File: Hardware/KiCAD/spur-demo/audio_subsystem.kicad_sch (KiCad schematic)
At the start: 16 parts, among them U3 MAX98357A, U4 LM393

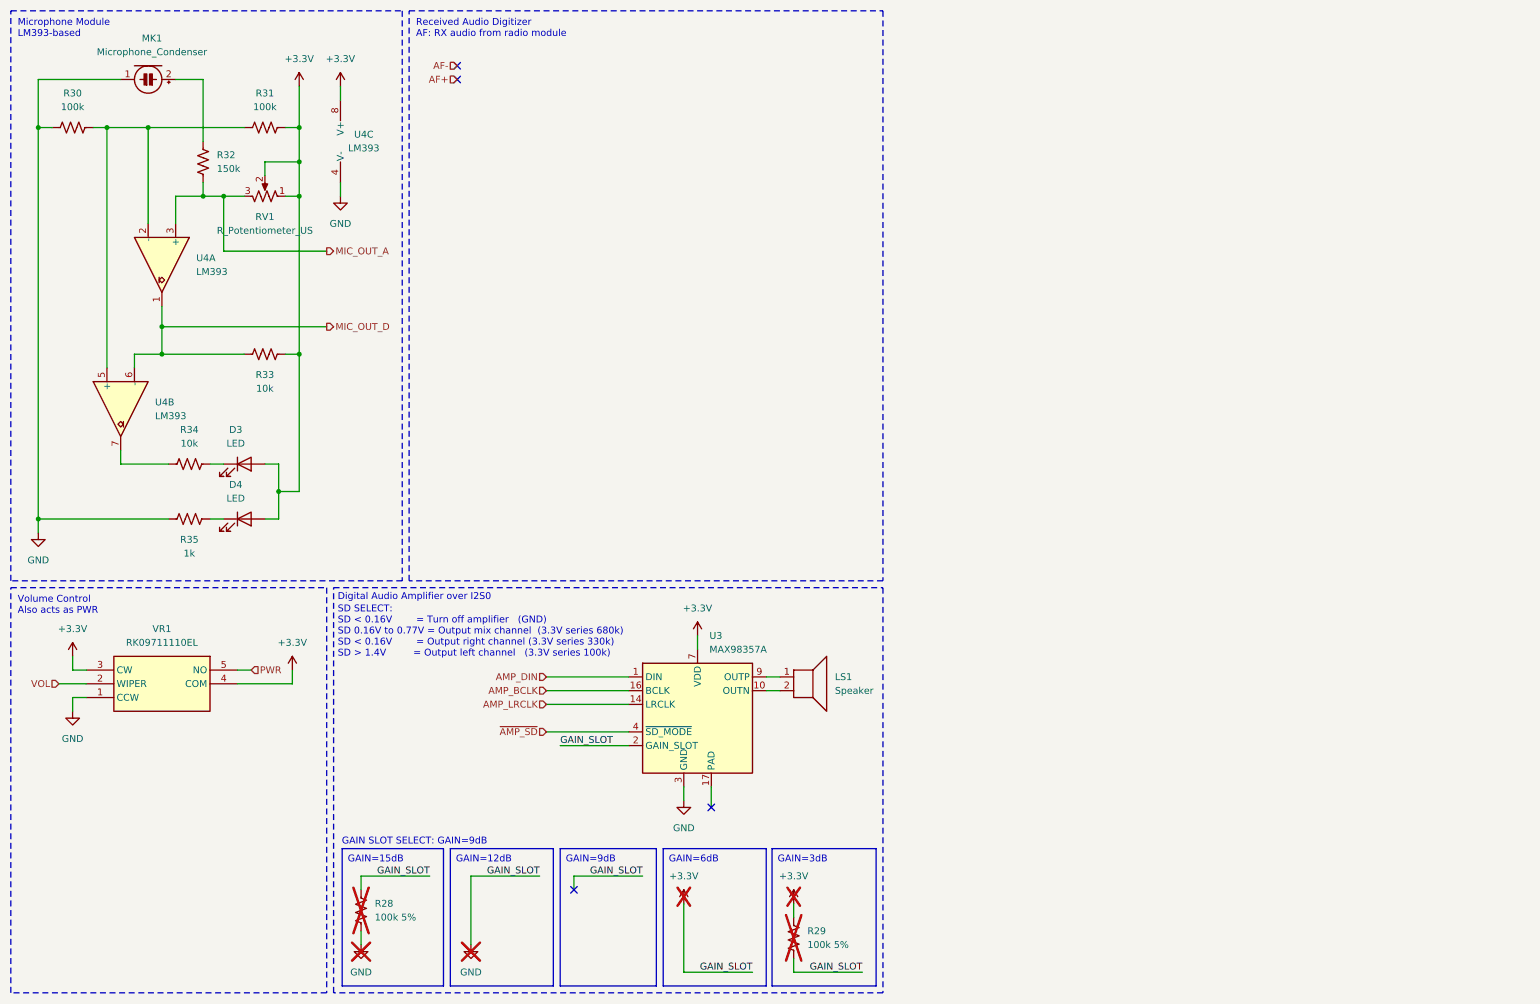
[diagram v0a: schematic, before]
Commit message: feat: configuration for audio amp through solder jumpers with set defaults
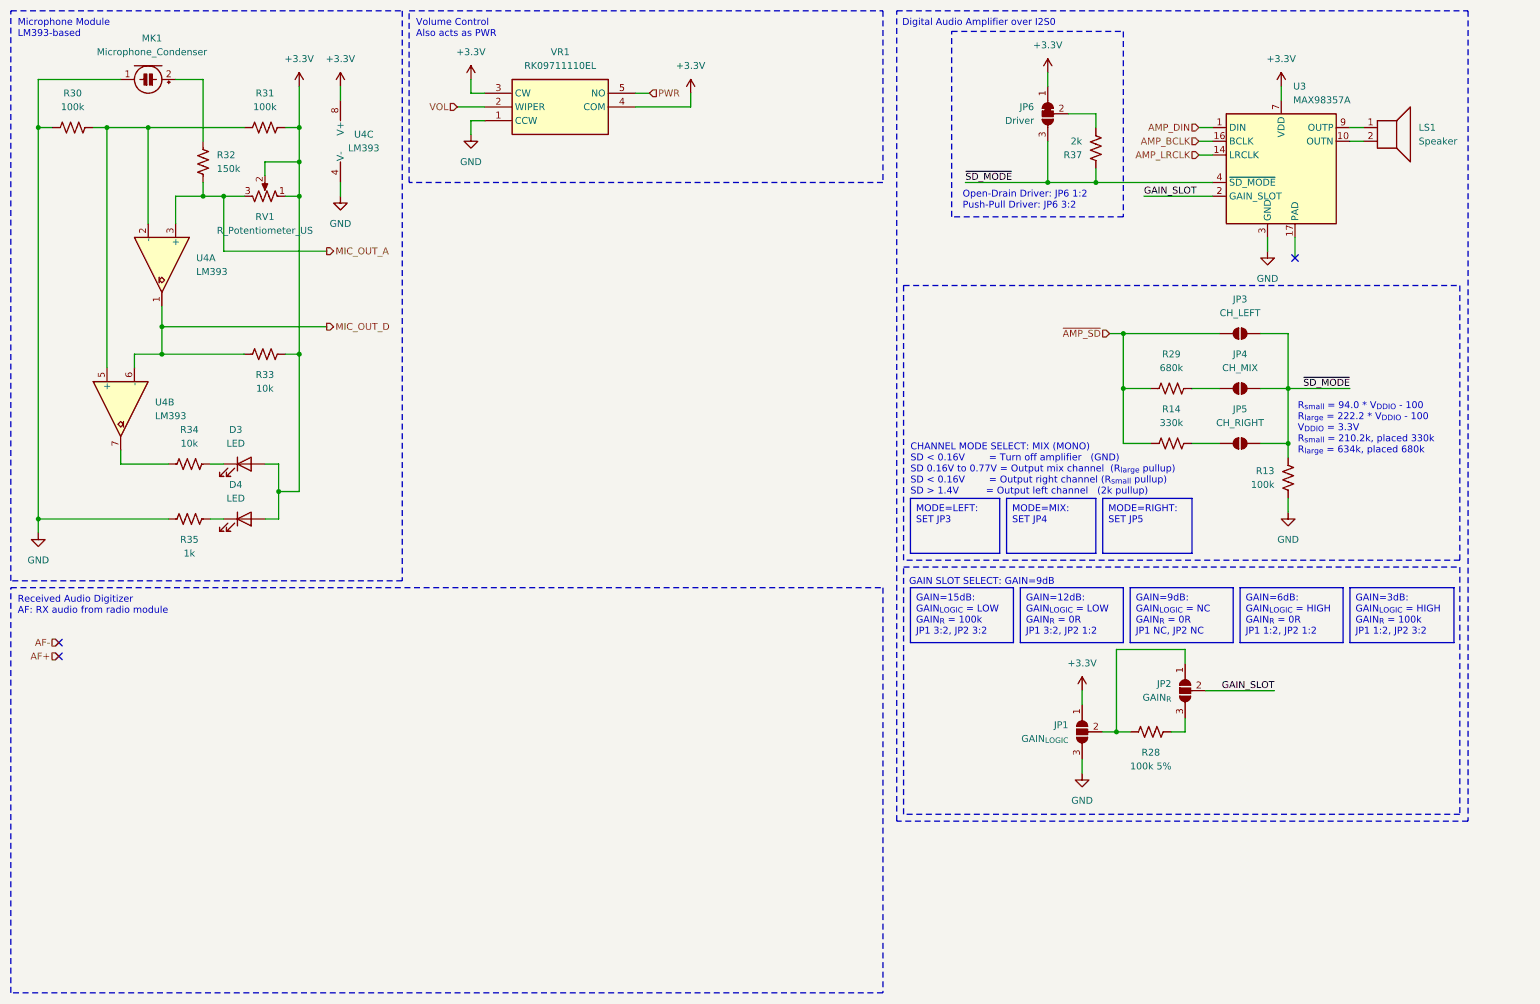
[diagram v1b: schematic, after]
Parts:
- added JP1: GAIN_{LOGIC}, symbol Jumper:SolderJumper_3_Open
- added JP2: GAIN_{R}, symbol Jumper:SolderJumper_3_Open
- added JP3: CH_LEFT, symbol Jumper:SolderJumper_2_Open
- added JP4: CH_MIX, symbol Jumper:SolderJumper_2_Open
- added JP5: CH_RIGHT, symbol Jumper:SolderJumper_2_Open
- added JP6: Driver, symbol Jumper:SolderJumper_3_Bridged12
- added R13: 100k, symbol Device:R_US
- added R14: 330k, symbol Device:R_US
- added R37: 2k, symbol Device:R_US
- R28: now fitted
- R29: value 100k 5% -> 680k; now fitted
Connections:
- net +3.3V: now also JP1.1 (A), JP6.1 (A); no longer MK1.1 (-), R28.1, R28.2, R29.1, R29.2, R30.2, R35.2, U3.11 (GND), U3.15 (GND), U3.2 (GAIN_SLOT), U3.3 (GND), U4.4 (V-), VR1.1 (CCW)
- net ~{AMP_SD}: now also R29.2, JP3.1 (A), R14.1; no longer U3.4 (~{SD_MODE})
- new net: JP6.2 (C), R37.1
- new net: JP4.1 (A), R29.1
- new net: JP1.2 (C), JP2.1 (A), R28.1
- new net: JP5.1 (A), R14.2
- new net: JP2.3 (B), R28.2
- new net GAIN_SLOT: JP2.2 (C), U3.2 (GAIN_SLOT)
- new net GND: JP1.3 (B), MK1.1 (-), R13.1, R30.2, R35.2, U3.11 (GND), U3.15 (GND), U3.3 (GND), U4.4 (V-), VR1.1 (CCW)
- new net ~{SD_MODE}: JP3.2 (B), JP4.2 (B), JP5.2 (B), JP6.3 (B), R13.2, R37.2, U3.4 (~{SD_MODE})
- no-connect marks 4 -> 3
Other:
- note added: "CHANNEL MODE SELECT: MIX (MONO) SD < 0.16V = Turn off amplifier (GND) SD 0.16V to 0.77V = Output mix channel (R_{large} pullup) SD < 0.16V = Output right channel (R_{small} pullup) SD > 1.4V = Output left channel (2k pullup)"
- note added: "Open-Drain Driver: JP6 1:2 Push-Pull Driver: JP6 3:2"
- note added: "R_{small} = 94.0 * V_{DDIO} - 100 R_{large} = 222.2 * V_{DDIO} - 100 V_{DDIO} = 3.3V R_{small} = 210.2k, placed 330k R_{large} = 634k, placed 680k"
- note removed: "SD SELECT: SD < 0.16V = Turn off amplifier (GND) SD 0.16V to 0.77V = Output mix channel (3.3V series 680k) SD < 0.16V = Output right channel (3.3V series 330k) SD > 1.4V = Output left channel (3.3V series 100k)"
- moved on the sheet: LS1, U3, VR1
